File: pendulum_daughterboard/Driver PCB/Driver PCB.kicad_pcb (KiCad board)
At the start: 2 copper layers, 32 parts, among them IC1 AND GATES, IC2 NAND (Used as AND), IC3 NAND (Used as Inverter), IC4 OR, J1 AVR-ISP-6, J2 Conn_01x02_Female, J4 Conn_01x04, J5 GND, J7 5V, Q1 BC557, Q2 BC547, SW1 SW_Push, U10 ATtiny85-20S

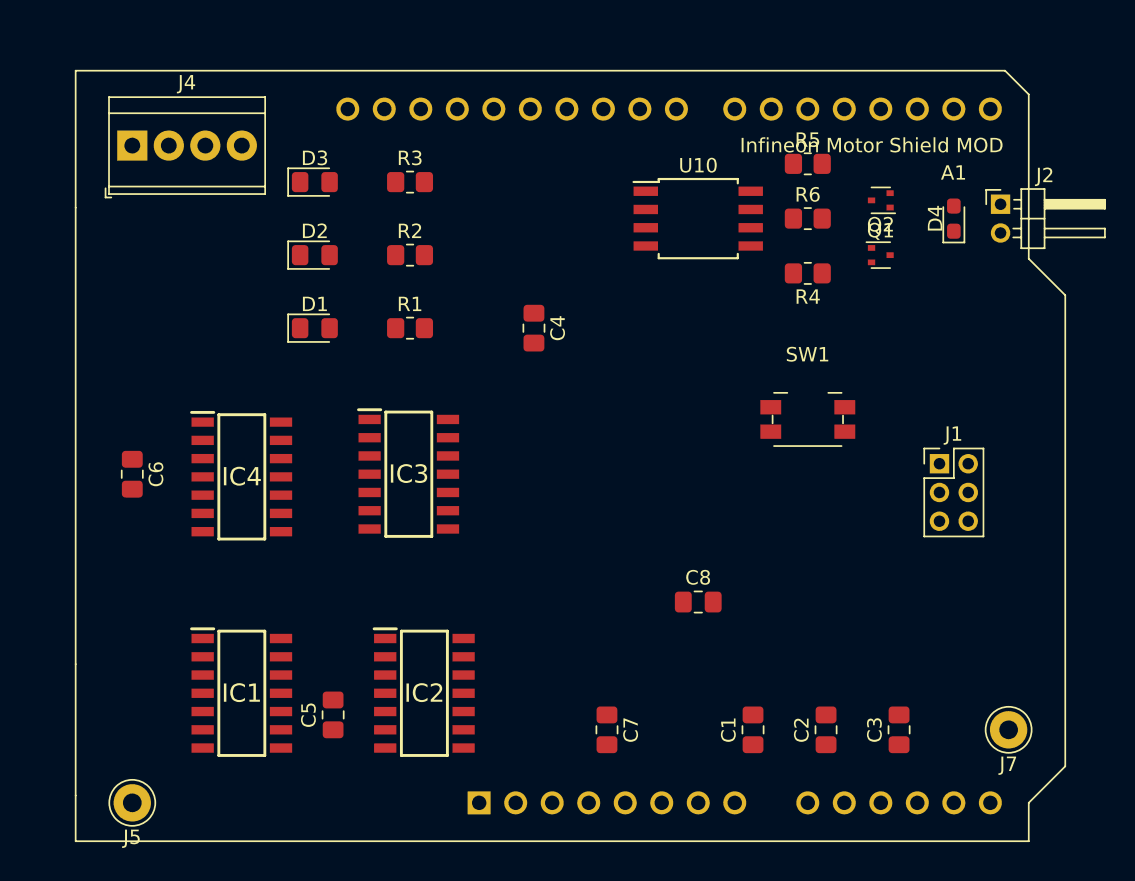
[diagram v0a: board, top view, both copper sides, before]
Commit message: Today's Progress on the PCB
22/06/22
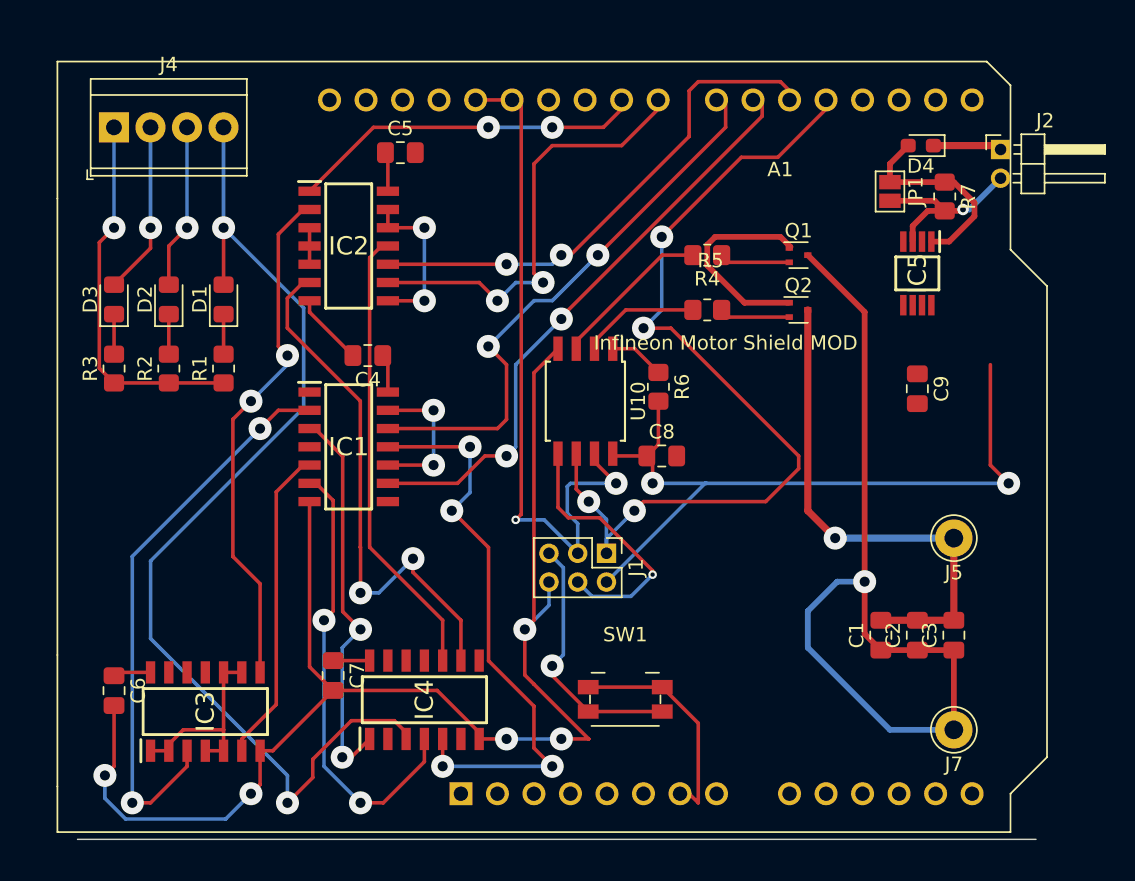
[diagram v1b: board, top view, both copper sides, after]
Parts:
- added C9: 0.1uF, Capacitor_SMD:C_0805_2012Metric_Pad1.18x1.45mm_HandSolder, F.Cu at (151.1, 77.9)
- added IC5: MAX9928FAUA+, Sensor_Current:SOP65P490X110-8N, F.Cu at (151.1, 69.8)
- added JP1: Shunt Bypass, Jumper:SolderJumper-2_P1.3mm_Open_Pad1.0x1.5mm, F.Cu at (149.2, 64.2)
- added R7: 10R, Resistor_SMD:R_0805_2012Metric_Pad1.20x1.40mm_HandSolder, F.Cu at (153.0, 64.5)
- D4: value D -> 1N4002
- J2: value Conn_01x02_Female -> Coil
- J5: value GND -> DRIVE_GND
- J7: value 5V -> DRIVE_5V_IN
- moved J5 60.0 mm to (153.7, 88.3)
- moved C5 39.4 mm to (115.2, 61.5), turned to 0 degrees
- moved IC2 31.6 mm to (111.6, 67.9)
- moved R3 24.3 mm to (95.2, 76.5), turned to 90 degrees
- moved J1 24.0 mm to (129.5, 89.3), turned to -90 degrees
- moved SW1 23.2 mm to (130.8, 99.5)
- moved IC3 21.7 mm to (101.6, 100.3), turned to 90 degrees
- moved IC4 20.0 mm to (116.8, 99.5), turned to 90 degrees
- moved C7 19.4 mm to (110.5, 97.8)
- moved IC1 18.7 mm to (111.6, 81.9)
- moved R2 18.5 mm to (99.1, 76.5), turned to 90 degrees
- moved D3 16.2 mm to (95.2, 71.7), turned to 90 degrees
- moved R6 15.6 mm to (133.1, 77.7), turned to -90 degrees
- moved C6 15.1 mm to (95.2, 98.9)
- moved U10 14.9 mm to (128.0, 78.7), turned to -90 degrees
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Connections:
- net DRIVE renamed DRIVE_INPUT
- net LOAD renamed LOAD_INPUT
- A1 pad 10: unconnected-(A1-Pad10) -> CURRENT_SIGN_OUT
- A1 pad 5: unconnected-(A1-Pad5) -> D_5V
- A1 pad 7: unconnected-(A1-Pad7) -> D_GND
- A1 pad 9: unconnected-(A1-Pad9) -> CURRENT_SENSE_OUT
- C1 pad 1: 5V -> DRIVE_5V
- C1 pad 2: GND -> DRIVE_GND
- C2 pad 1: 5V -> DRIVE_5V
- C2 pad 2: GND -> DRIVE_GND
- C3 pad 1: 5V -> DRIVE_5V
- C3 pad 2: GND -> DRIVE_GND
- C4 pad 1: 5V -> D_5V
- C4 pad 2: GND -> D_GND
- C5 pad 1: 5V -> D_5V
- C5 pad 2: GND -> D_GND
- C6 pad 1: 5V -> D_5V
- C6 pad 2: GND -> D_GND
- C7 pad 1: 5V -> D_5V
- C7 pad 2: GND -> D_GND
- C8 pad 1: 5V -> D_5V
- C8 pad 2: GND -> D_GND
- D4 pad 1: GND -> DRIVE_GND
- D4 pad 2: Net-(D4-Pad2) -> Net-(R7-Pad1)
- IC1 pad 10: /LED_Circit/STUDENT_ENABLE -> STUDENT_ENABLE
- IC1 pad 13: ENABLE -> STUDENT_ENABLE
- IC1 pad 14: 5V -> D_5V
- IC1 pad 7: GND -> D_GND
- IC2 pad 10: /LED_Circit/STUDENT_ENABLE -> STUDENT_ENABLE
- IC2 pad 14: 5V -> D_5V
- IC2 pad 7: GND -> D_GND
- IC3 pad 1: /LED_Circit/STUDENT_ENABLE -> STUDENT_ENABLE
- IC3 pad 10: /LED_Circit/STUDENT_ENABLE -> STUDENT_ENABLE
- IC3 pad 14: 5V -> D_5V
- IC3 pad 2: /LED_Circit/STUDENT_ENABLE -> STUDENT_ENABLE
- IC3 pad 4: /LED_Circit/STUDENT_ENABLE -> STUDENT_ENABLE
- IC3 pad 5: /LED_Circit/STUDENT_ENABLE -> STUDENT_ENABLE
- IC3 pad 7: GND -> D_GND
- IC3 pad 9: /LED_Circit/STUDENT_ENABLE -> STUDENT_ENABLE
- IC4 pad 14: 5V -> D_5V
- IC4 pad 7: GND -> D_GND
- J1 pad 2: 5V -> D_5V
- J1 pad 6: GND -> D_GND
- J2 pad 1: Net-(D4-Pad2) -> DRIVE_GND
- J2 pad 2: GND -> Net-(R7-Pad2)
- J4 pad 1: OR_OUT_1 -> D_GND
- J4 pad 2: OR_OUT_2 -> OR_OUT_3
- J4 pad 3: OR_OUT_3 -> OR_OUT_2
- J4 pad 4: GND -> OR_OUT_1
- J5 pad 1: GND -> DRIVE_GND
- J7 pad 1: 5V -> DRIVE_5V
- Q1 pad 1: Net-(D4-Pad2) -> Net-(R7-Pad1)
- Q1 pad 3: 5V -> DRIVE_5V
- Q2 pad 1: Net-(D4-Pad2) -> Net-(R7-Pad1)
- Q2 pad 3: GND -> DRIVE_GND
- R1 pad 1: GND -> D_GND
- R2 pad 1: GND -> D_GND
- R3 pad 1: GND -> D_GND
- R6 pad 2: 5V -> D_5V
- SW1 pad 1: GND -> D_GND
- U10 pad 4: GND -> D_GND
- U10 pad 8: 5V -> D_5V
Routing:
- net D_GND: track 0.00 -> 142.6 mm, vias 0 -> 6
- net OR_OUT_1: track 0.00 -> 73.8 mm, vias 0 -> 2
- net D_5V: track 0.00 -> 62.7 mm, vias 0 -> 2
- net LOAD_INPUT: track 0.00 -> 62.5 mm, vias 0 -> 4
- net STUDENT_ENABLE: track 0.00 -> 60.3 mm, vias 0 -> 4
- net DRIVE_5V: track 0.00 -> 60.1 mm, vias 0 -> 1
- net DRIVE_INPUT: track 0.00 -> 48.3 mm, vias 0 -> 2
- net STU_LED_1: track 0.00 -> 41.2 mm, vias 0 -> 2
- net AND_STU_LED_2: track 0.00 -> 40.9 mm, vias 0 -> 4
- net DRIVE_GND: track 0.00 -> 40.5 mm, vias 0 -> 1
- net INV_1: track 0.00 -> 39.6 mm, vias 0 -> 2
- net STU_LED_2: track 0.00 -> 38.9 mm, vias 0 -> 2
- net AND_SUP_LED_3: track 0.00 -> 37.7 mm, vias 0 -> 2
- net INV_3: track 0.00 -> 36.0 mm, vias 0 -> 2
- net AND_STU_LED_3: track 0.00 -> 31.7 mm
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
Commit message: changes
11.50
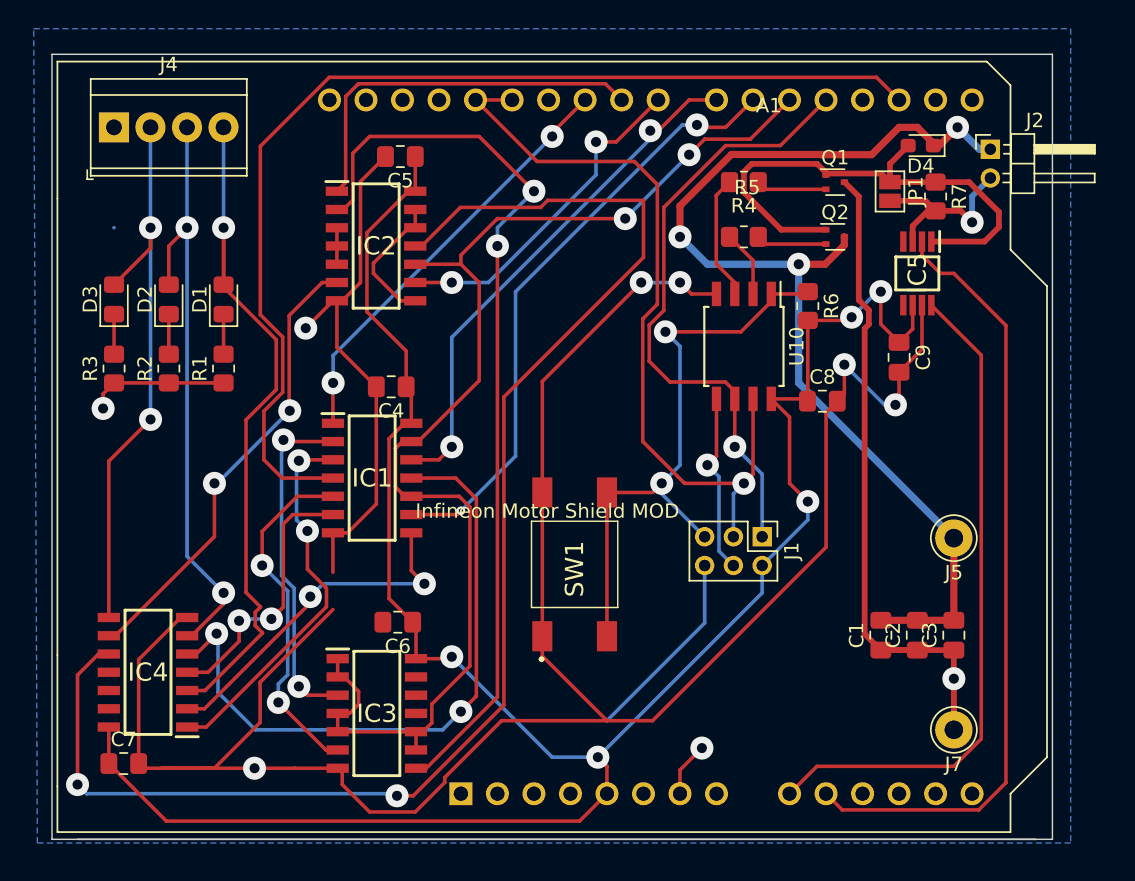
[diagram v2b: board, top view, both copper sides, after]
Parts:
- SW1: footprint Button_Switch_SMD:Panasonic_EVQPUK_EVQPUB -> Button_Switch_SMD:13019319
- moved C6 20.3 mm to (115.0, 94.1), turned to 180 degrees
- moved IC4 19.3 mm to (97.6, 97.6), turned to 180 degrees
- moved C7 15.8 mm to (95.9, 103.9), turned to 0 degrees
- moved IC3 11.9 mm to (113.5, 100.5), turned to 0 degrees
- moved R6 11.8 mm to (143.5, 72.1)
- moved C8 11.8 mm to (144.5, 78.7)
- moved U10 11.7 mm to (139.1, 74.9)
- moved J1 10.9 mm to (140.3, 88.2)
- moved SW1 9.24 mm to (127.3, 90.9), turned to 90 degrees
- moved R4 5.68 mm to (139.1, 63.5)
- moved R5 5.68 mm to (139.1, 67.3)
- moved Q1 5.68 mm to (145.4, 63.5)
- moved Q2 5.68 mm to (145.4, 67.3)
- moved C4 2.71 mm to (114.5, 77.7)
- moved IC1 2.71 mm to (113.2, 84.1)
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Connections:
- SW1 pad 2: Net-(J1-Pad5) -> D_GND
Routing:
- net D_5V: track 62.7 -> 151.3 mm, vias 2 -> 5
- net D_GND: track 142.6 -> 219.3 mm, vias 6 -> 8
- net SUP_LED_2: track 0.00 -> 75.4 mm
- net AND_STU_LED_3: track 31.7 -> 99.3 mm, vias 0 -> 2
- net CURRENT_SIGN_OUT: track 0.00 -> 54.4 mm
- net CURRENT_SENSE_OUT: track 0.00 -> 46.5 mm
- net DRIVE_GND: track 40.5 -> 75.7 mm, vias 1 -> 3
- net OR_OUT_2: track 11.5 -> 42.1 mm, vias 1 -> 2
- net SUP_LED_1: track 0.00 -> 29.8 mm, vias 0 -> 2
- net OR_OUT_3: track 12.0 -> 40.3 mm, vias 1 -> 2
- net INV_3: track 36.0 -> 63.2 mm
- net STUDENT_ENABLE: track 60.3 -> 87.2 mm, vias 4 -> 2
- net OR_OUT_1: track 73.8 -> 49.2 mm, vias 2 -> 1
- net AND_STU_LED_1: track 0.00 -> 24.3 mm, vias 0 -> 2
- net Net-(J1-Pad5): track 21.8 -> 41.9 mm, vias 1 -> 2
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- added copper zone on B.Cu, net D_GND
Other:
- board outline added: 69.6 x 54.6 mm

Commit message: Changes to the PCB
23/06/2022
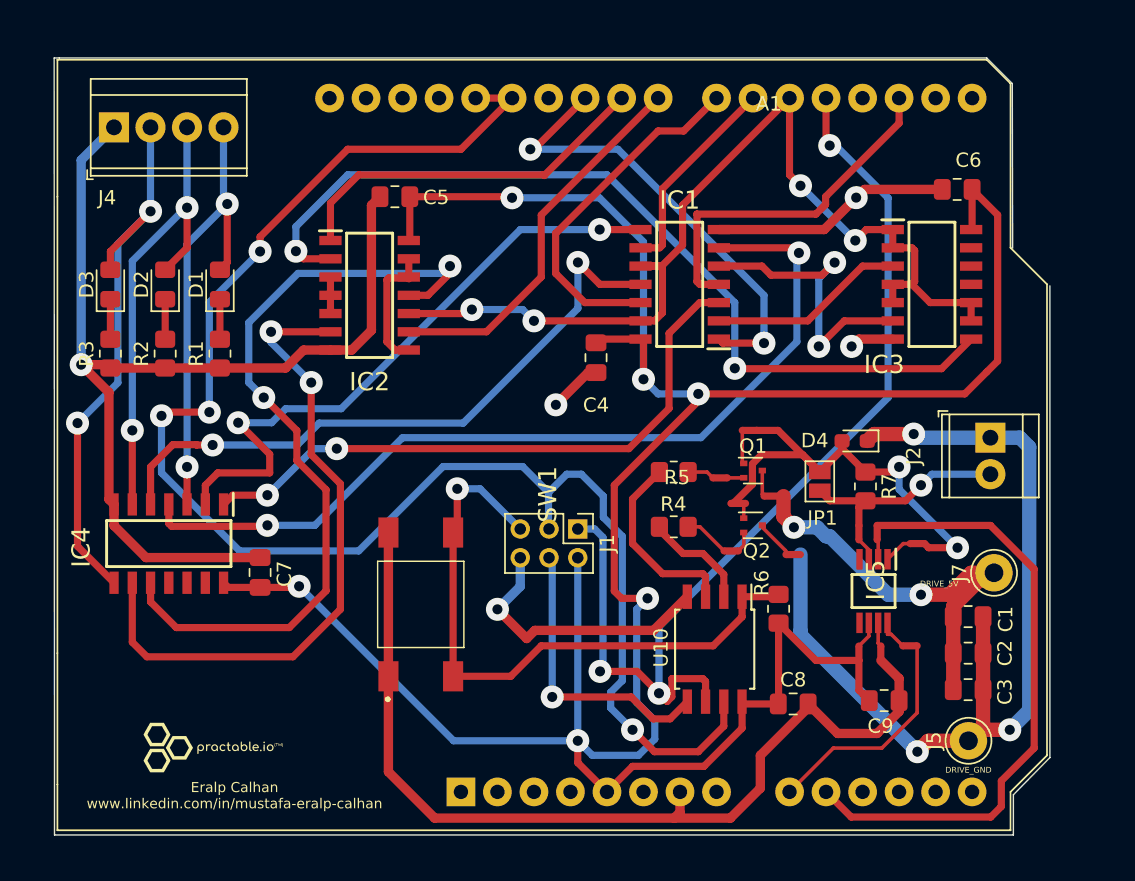
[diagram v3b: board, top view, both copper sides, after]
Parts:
- added G***: LOGO, 000_Graphics_Immo:practactable.io_text_10x4, F.Cu at (102.1, 102.9)
- added NT1: NetTie_2, NetTie:NetTie-2_SMD_Pad0.5mm, F.Cu at (147.1, 96.3)
- added NT10: NetTie_2, NetTie:NetTie-2_SMD_Pad0.5mm, F.Cu at (138.2, 89.2)
- added NT11: NetTie_2, NetTie:NetTie-2_SMD_Pad0.5mm, F.Cu at (138.7, 85.9)
- added NT12: NetTie_2, NetTie:NetTie-2_SMD_Pad0.5mm, F.Cu at (142.5, 89.4)
- added NT2: NetTie_2, NetTie:NetTie-2_SMD_Pad0.5mm, F.Cu at (148.6, 96.3)
- added NT3: NetTie_2, NetTie:NetTie-2_SMD_Pad0.5mm, F.Cu at (148.3, 87.9)
- added NT4: NetTie_2, NetTie:NetTie-2_SMD_Pad0.5mm, F.Cu at (147.1, 87.9)
- added NT5: NetTie_2, NetTie:NetTie-2_SMD_Pad0.5mm, F.Cu at (151.1, 88.6)
- added NT6: NetTie_2, NetTie:NetTie-2_SMD_Pad0.5mm, F.Cu at (150.6, 95.8)
- added NT7: NetTie_2, NetTie:NetTie-2_SMD_Pad0.5mm, F.Cu at (141.0, 85.3)
- added NT8: NetTie_2, NetTie:NetTie-2_SMD_Pad0.5mm, F.Cu at (137.4, 84.1)
- added NT9: NetTie_2, NetTie:NetTie-2_SMD_Pad0.5mm, F.Cu at (139.5, 80.8)
- J2: footprint Connector_PinHeader_2.00mm:PinHeader_1x02_P2.00mm_Horizontal -> TerminalBlock_TE-Connectivity:TerminalBlock_TE_282834-2_1x02_P2.54mm_Horizontal
- moved C6 49.2 mm to (153.9, 64.0)
- moved IC3 48.8 mm to (152.1, 70.6)
- moved IC1 25.3 mm to (134.6, 70.6), turned to 180 degrees
- moved C9 23.9 mm to (148.8, 99.6), turned to 0 degrees
- moved IC5 22.3 mm to (148.1, 91.9)
- moved C8 21.2 mm to (142.5, 99.8)
- moved R6 21.2 mm to (141.5, 93.2)
- moved U10 21.2 mm to (137.0, 96.0)
- moved D4 21.1 mm to (146.8, 81.5)
- moved Q1 20.9 mm to (139.7, 83.6)
- moved Q2 20.9 mm to (139.7, 87.4)
- moved R7 20.8 mm to (147.5, 84.7)
- moved R4 20.8 mm to (134.2, 83.7)
- moved R5 20.8 mm to (134.2, 87.5)
- moved JP1 20.8 mm to (144.3, 84.3)
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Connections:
- D4 pad 2: Net-(R7-Pad1) -> Net-(D4-Pad2)
- IC5 pad 1: Net-(R7-Pad1) -> Net-(IC5-Pad1)
- IC5 pad 2: CURRENT_SIGN_OUT -> Net-(IC5-Pad2)
- IC5 pad 3: Net-(R7-Pad2) -> Net-(IC5-Pad3)
- IC5 pad 6: D_5V -> Net-(IC5-Pad6)
- IC5 pad 7: D_GND -> Net-(IC5-Pad7)
- IC5 pad 8: CURRENT_SENSE_OUT -> Net-(IC5-Pad8)
- J2 pad 2: Net-(R7-Pad2) -> Net-(J2-Pad2)
- JP1 pad 1: Net-(R7-Pad1) -> Net-(D4-Pad2)
- JP1 pad 2: Net-(R7-Pad2) -> Net-(J2-Pad2)
- Q1 pad 1: Net-(R7-Pad1) -> Net-(Q1-Pad1)
- Q1 pad 3: DRIVE_5V -> Net-(Q1-Pad3)
- Q2 pad 1: Net-(R7-Pad1) -> Net-(Q2-Pad1)
- Q2 pad 3: DRIVE_GND -> Net-(Q2-Pad3)
- R4 pad 1: Net-(Q1-Pad2) -> Net-(R4-Pad1)
- R5 pad 1: Net-(Q2-Pad2) -> Net-(R5-Pad1)
- R7 pad 1: Net-(R7-Pad1) -> Net-(D4-Pad2)
- R7 pad 2: Net-(R7-Pad2) -> Net-(J2-Pad2)
- SW1 pad 2: D_GND -> Net-(J1-Pad5)
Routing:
- net DRIVE_INPUT: track 54.3 -> 112.6 mm, vias 1 -> 4
- net SUP_LED_2: track 75.4 -> 25.0 mm
- net AND_STU_LED_3: track 99.3 -> 55.8 mm
- net AND_SUP_LED_2: track 18.9 -> 62.4 mm
- net D_5V: track 151.3 -> 190.7 mm, vias 5 -> 6
- net D_GND: track 219.3 -> 180.4 mm, vias 8 -> 5
- net Net-(R7-Pad1): track 37.0 -> 0.00 mm
- net Net-(D4-Pad2): track 0.00 -> 32.3 mm, vias 0 -> 2
- net CURRENT_SENSE_OUT: track 46.5 -> 15.8 mm
- net LOAD_INPUT: track 43.2 -> 72.5 mm, vias 1 -> 3
- net STU_LED_1: track 42.6 -> 14.4 mm, vias 2 -> 0
- net DRIVE_5V: track 50.1 -> 28.6 mm, vias 1 -> 2
- net AND_STU_LED_1: track 24.3 -> 44.1 mm
- net STUDENT_ENABLE: track 87.2 -> 68.4 mm, vias 2 -> 4
- net OR_OUT_1: track 49.2 -> 32.3 mm, vias 1 -> 2
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- removed copper zone on B.Cu, net D_GND
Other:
- board size 69.6 x 54.6 mm -> 69.3 x 54.1 mm
- board text added: "DRIVE_5V"
- board text added: "DRIVE_GND"
- board text added: "Eralp Calhan www.linkedin.com/in/mustafa-eralp-calhan"
